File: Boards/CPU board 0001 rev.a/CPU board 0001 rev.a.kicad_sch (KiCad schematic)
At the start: 78 parts, among them J1 CEC card edge connector large, U10 7432, U11 7442, U12 7406, U13 7406, U14 7442, U15 7442, U16 M8216, U17 M8216, U18 6532, U19 6532, U20 2708, U21 2708, U22 2708, U23 74367, U24 74367, U25 6502, U5 74367, U6 7414, U7 LM7905_TO220, U8 7406, U9 7408, Y1 1Mhz

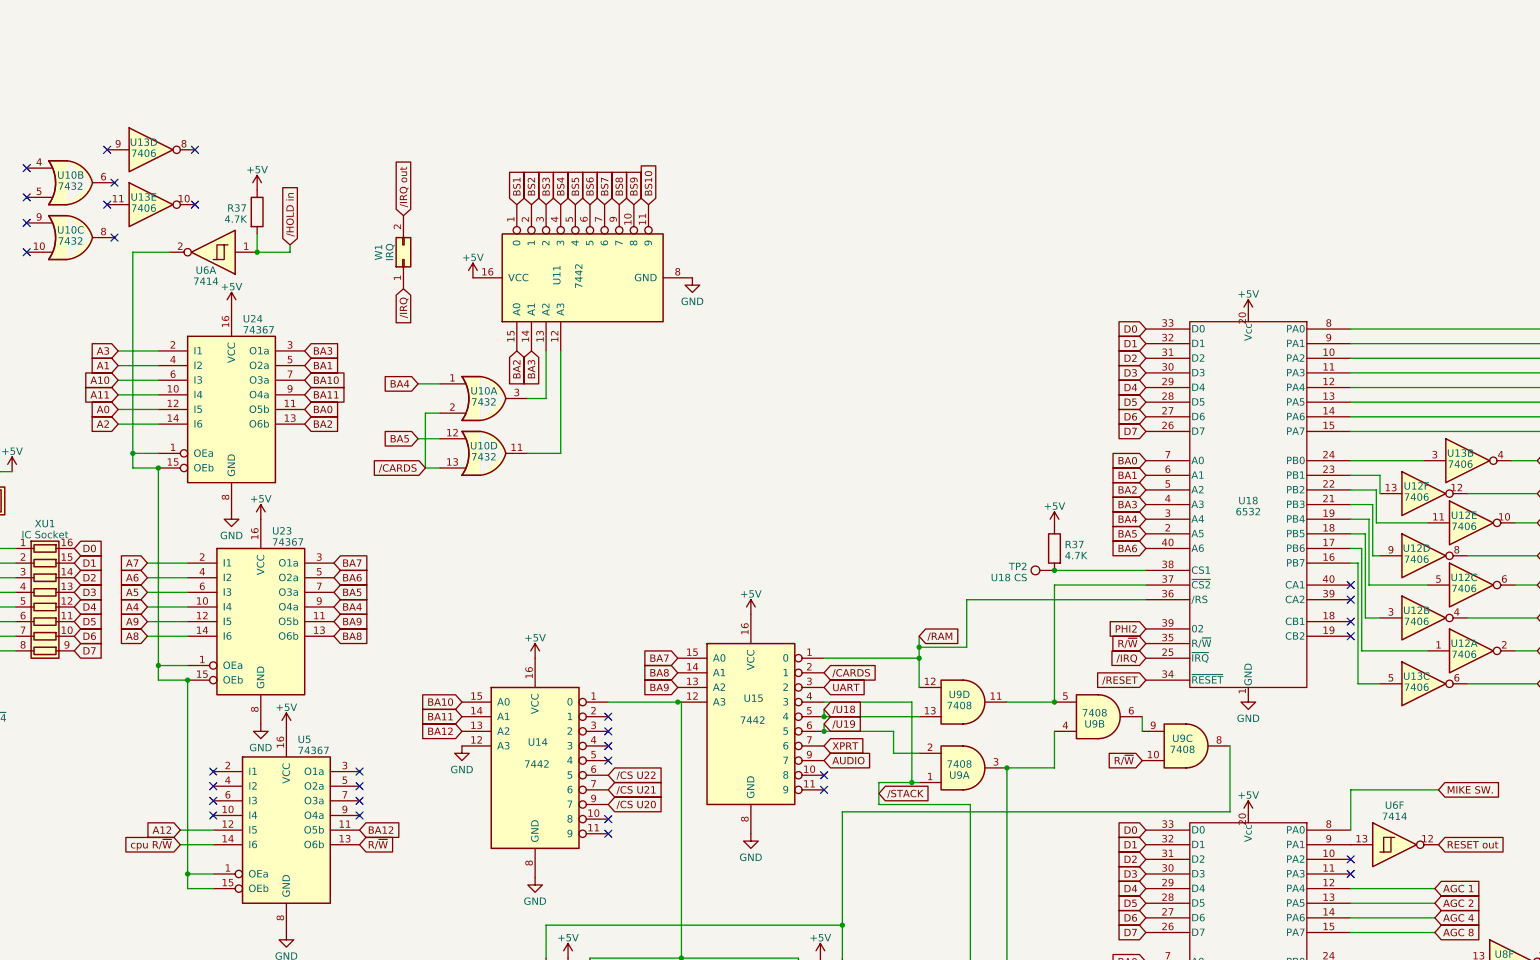
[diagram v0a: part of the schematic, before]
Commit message: continued routing
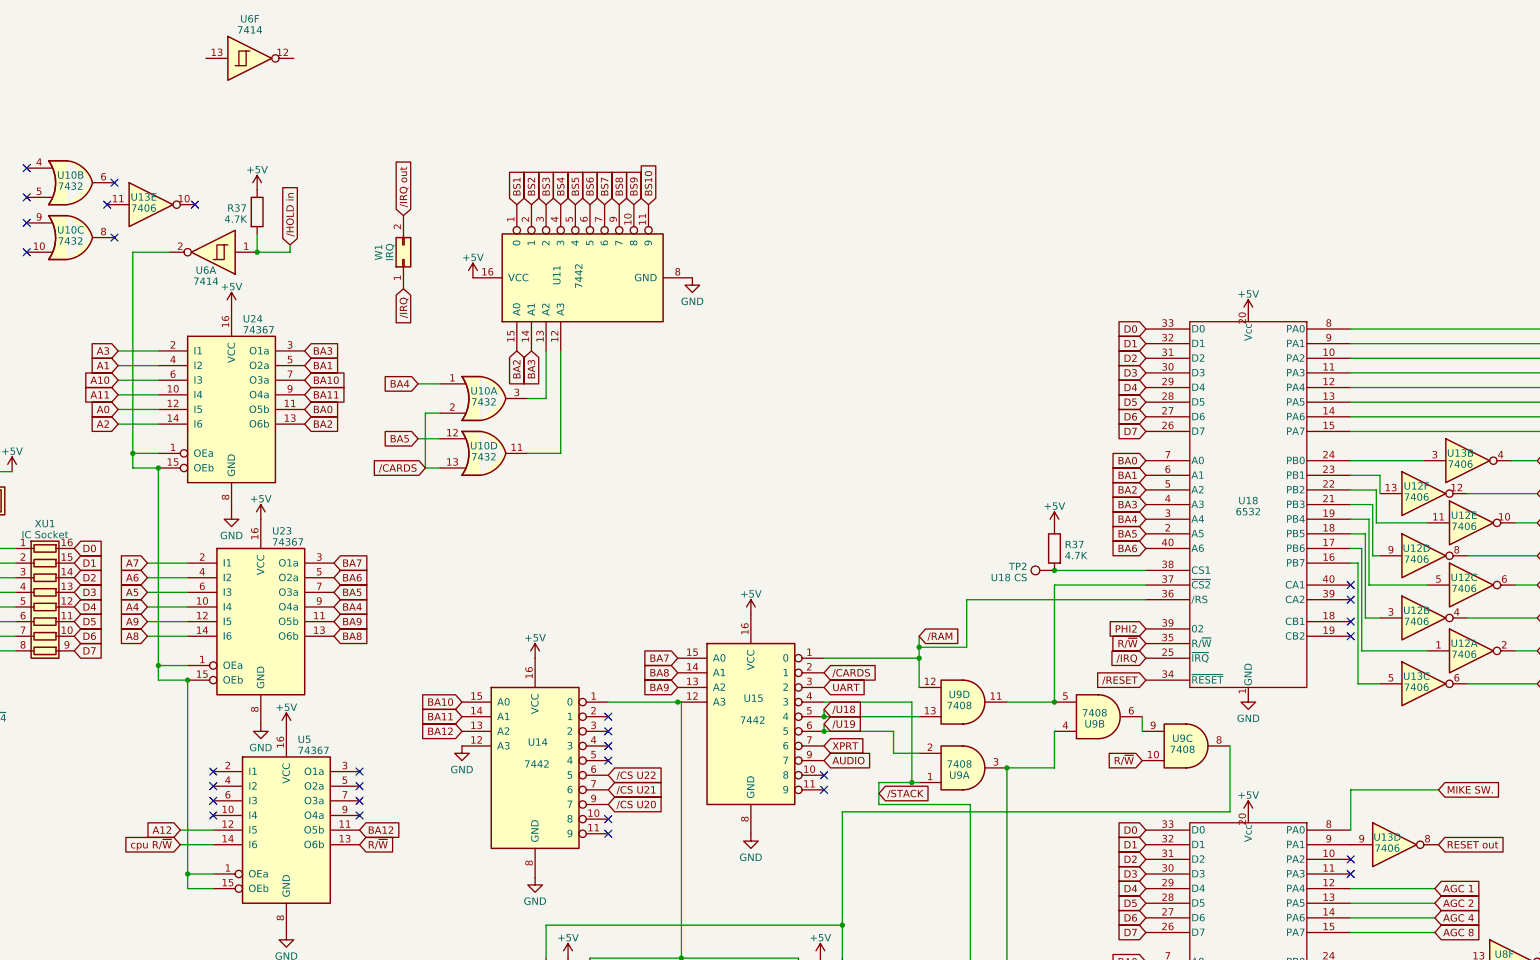
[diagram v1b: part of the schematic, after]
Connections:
- net RESET out: now also U13.8; no longer U6.12
- net at U6.13: no longer U19.9 (PA1)
- net at U13.9: now also U19.9 (PA1)
- net at U18.18 (PB5): now also U12.3
- no-connect marks 126 -> 124
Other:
- moved on the sheet: U13D
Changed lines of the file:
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@@
   (no_connect (at 173.355 203.835))
   (no_connect (at 44.45 154.94))
-  (no_connect (at 218.44 16.51))
   (no_connect (at 170.815 193.675))
   (no_connect (at 31.75 25.4))
@@
   (no_connect (at 31.75 127))
   (no_connect (at 157.48 145.415))
-  (no_connect (at 203.2 16.51))
   (no_connect (at 189.23 24.765))
   (no_connect (at 259.715 204.47))
@@
     )
   )
+  (symbol (lib_id "74xx:74LS14") (at 227.965 0.635 0) (unit 6)
+    (in_bom yes) (on_board yes) (dnp no) (fields_autoplaced)
+    (property "Reference" "U6" (at 227.965 -6.1849 0)
+      (effects (font (size 1.27 1.27)))
+    )
+    (property "Value" "7414" (at 227.965 -4.2639 0)
+      (effects (font (size 1.27 1.27)))
+    )
+    (property "Footprint" "Package_DIP:DIP-14_W7.62mm" (at 227.965 0.635 0)
+      (effects (font (size 1.27 1.27)) hide)
+    )
+    (property "Datasheet" "http://www.ti.com/lit/gpn/sn74LS14" (at 227.965 0.635 0)
+      (effects (font (size 1.27 1.27)) hide)
+    )
+    (pin "1")
+    (pin "2")
+    (pin "3")
+    (pin "4")
+    (pin "5")
+    (pin "6")
+    (pin "8")
+    (pin "9")
+    (pin "10")
+    (pin "11")
+    (pin "12")
+    (pin "13")
+    (pin "14")
+    (pin "7")
+    (instances
+      (project "CPU board 0001 rev.a"
+        (path "/972f3ffb-6bde-4480-8d3a-f1aadeb0cbf8"
+          (reference "U6") (unit 6)
+        )
+      )
+    )
+  )
   (symbol (lib_id "power:+5V") (at 277.495 104.775 0) (unit 1)
     (in_bom yes) (on_board yes) (dnp no) (fields_autoplaced)
@@
     )
   )
-  (symbol (lib_id "74xx:74LS14") (at 426.72 137.16 0) (unit 6)
-    (in_bom yes) (on_board yes) (dnp no) (fields_autoplaced)
-    (property "Reference" "U6" (at 426.72 130.3401 0)
-      (effects (font (size 1.27 1.27)))
-    )
-    (property "Value" "7414" (at 426.72 132.2611 0)
-      (effects (font (size 1.27 1.27)))
-    )
-    (property "Footprint" "Package_DIP:DIP-14_W7.62mm" (at 426.72 137.16 0)
-      (effects (font (size 1.27 1.27)) hide)
-    )
-    (property "Datasheet" "http://www.ti.com/lit/gpn/sn74LS14" (at 426.72 137.16 0)
-      (effects (font (size 1.27 1.27)) hide)
-    )
-    (pin "1")
-    (pin "2")
-    (pin "3")
-    (pin "4")
-    (pin "5")
-    (pin "6")
-    (pin "8")
-    (pin "9")
-    (pin "10")
-    (pin "11")
-    (pin "12")
-    (pin "13")
-    (pin "14")
-    (pin "7")
-    (instances
-      (project "CPU board 0001 rev.a"
-        (path "/972f3ffb-6bde-4480-8d3a-f1aadeb0cbf8"
-          (reference "U6") (unit 6)
-        )
-      )
-    )
-  )
   (symbol (lib_id "power:+5V") (at 178.435 21.59 0) (unit 1)
     (in_bom yes) (on_board yes) (dnp no) (fields_autoplaced)
@@
     )
   )
-  (symbol (lib_id "74xx:74LS06") (at 210.82 16.51 0) (unit 4)
+  (symbol (lib_id "74xx:74LS06") (at 426.72 137.16 0) (unit 4)
     (in_bom yes) (on_board yes) (dnp no)
-    (property "Reference" "U13" (at 209.55 15.224 0)
+    (property "Reference" "U13" (at 425.45 135.874 0)
       (effects (font (size 1.27 1.27)))
     )
-    (property "Value" "7406" (at 209.55 17.145 0)
+    (property "Value" "7406" (at 425.45 137.795 0)
       (effects (font (size 1.27 1.27)))
     )
-    (property "Footprint" "Package_DIP:DIP-14_W7.62mm" (at 210.82 16.51 0)
+    (property "Footprint" "Package_DIP:DIP-14_W7.62mm" (at 426.72 137.16 0)
       (effects (font (size 1.27 1.27)) hide)
     )
-    (property "Datasheet" "http://www.ti.com/lit/gpn/sn74LS06" (at 210.82 16.51 0)
+    (property "Datasheet" "http://www.ti.com/lit/gpn/sn74LS06" (at 426.72 137.16 0)
       (effects (font (size 1.27 1.27)) hide)
     )
